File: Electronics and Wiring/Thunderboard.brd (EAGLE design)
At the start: 84.1 x 54.6 mm, 33 parts, among them Q1 TIP120, Q2 TIP120, Q3 TIP120, T1 2n2222

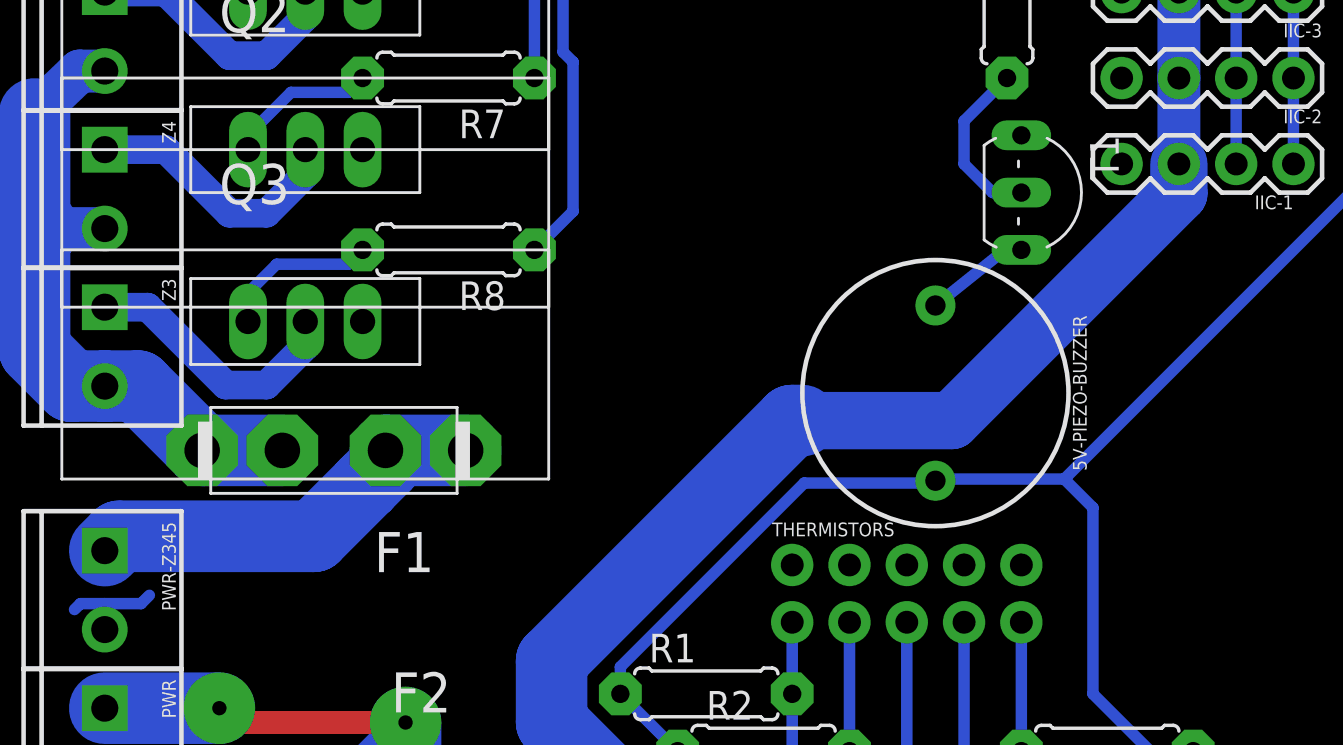
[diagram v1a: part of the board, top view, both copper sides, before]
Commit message: Updating electronics files
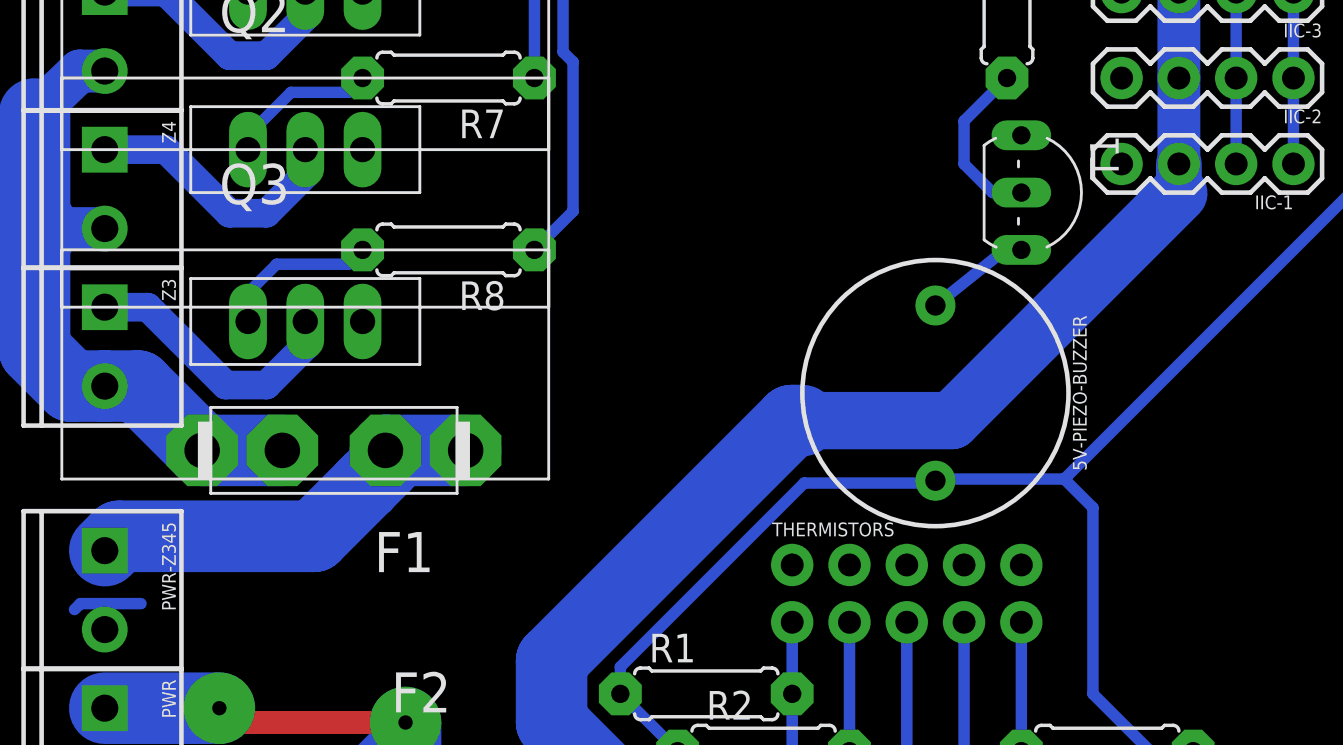
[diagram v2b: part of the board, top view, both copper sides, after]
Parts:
- R9: value 1K -> 3K
- T1: value 2n2222 -> PN2222A
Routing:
- net GND: track 4.74 -> 4.21 mm
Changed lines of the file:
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@@
 <layer number="19" name="Unrouted" color="6" fill="1" visible="no" active="yes"/>
 <layer number="20" name="Dimension" color="24" fill="1" visible="yes" active="yes"/>
-<layer number="21" name="tPlace" color="7" fill="1" visible="no" active="yes"/>
+<layer number="21" name="tPlace" color="7" fill="1" visible="yes" active="yes"/>
 <layer number="22" name="bPlace" color="7" fill="1" visible="no" active="yes"/>
 <layer number="23" name="tOrigins" color="15" fill="1" visible="no" active="yes"/>
@@
 <attribute name="VALUE" x="50.038" y="24.765" size="0.6096" layer="27" font="vector" ratio="20" rot="R270" align="top-center"/>
 </element>
-<element name="T1" library="transistor" library_urn="urn:adsk.eagle:library:402" package="TO92-EBC" package3d_urn="urn:adsk.eagle:package:29915/2" value="2n2222" x="49.53" y="33.655" smashed="yes" rot="R270">
+<element name="T1" library="transistor" library_urn="urn:adsk.eagle:library:402" package="TO92-EBC" package3d_urn="urn:adsk.eagle:package:29915/2" value="PN2222A" x="49.53" y="33.655" smashed="yes" rot="R270">
 <attribute name="NAME" x="51.308" y="36.195" size="1.27" layer="25" ratio="10" rot="R270"/>
 </element>
-<element name="R9" library="resistor - edit" package="0207/7" package3d_urn="urn:adsk.eagle:package:25942/1" value="1K" x="47.625" y="42.545" smashed="yes" rot="R270">
+<element name="R9" library="resistor - edit" package="0207/7" package3d_urn="urn:adsk.eagle:package:25942/1" value="3K" x="47.625" y="42.545" smashed="yes" rot="R270">
 <attribute name="NAME" x="49.022" y="45.085" size="1.27" layer="25" ratio="10" rot="R270"/>
 <attribute name="VALUE" x="47.0662" y="44.831" size="1.27" layer="27" ratio="10" rot="R270"/>
@@
 <wire x1="7.62" y1="14.28" x2="7.62" y2="15.4305" width="0.508" layer="16"/>
 <wire x1="7.62" y1="15.4305" x2="9.2282" y2="15.4305" width="0.508" layer="16"/>
-<wire x1="9.59885" y1="15.80115" x2="9.2282" y2="15.4305" width="0.508" layer="16"/>
 <wire x1="7.62" y1="15.4305" x2="6.5405" y2="15.4305" width="0.508" layer="16"/>
 <wire x1="6.5405" y1="15.4305" x2="6.27615" y2="15.16615" width="0.508" layer="16"/>
@@
 <wire x1="27.432" y1="12.8997" x2="38.0793" y2="23.547" width="3.175" layer="16"/>
 <wire x1="45.17055" y1="23.547" x2="55.245" y2="33.62145" width="2.54" layer="16"/>
-<wire x1="55.245" y1="33.62145" x2="55.245" y2="34.925" width="2.54" layer="16"/>
+<wire x1="55.245" y1="33.62145" x2="55.245" y2="34.925" width="2.032" layer="16"/>
 </signal>
 <signal name="D11">
